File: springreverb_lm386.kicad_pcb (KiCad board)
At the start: 2 copper layers, 65 x 54.7 mm, 50 parts, among them J1 IN, J10 To2, J13 FromGND, J14 From, J15 VR2_3, J16 VR2_3GND, J2 INGND, J3 GND, J4 Vin, J5 VR1_3, J6 VR1_2, J7 VR3_1, J8 ToGND, J9 To, U1 TL072, U2 TC1044S, U3 4556ADD

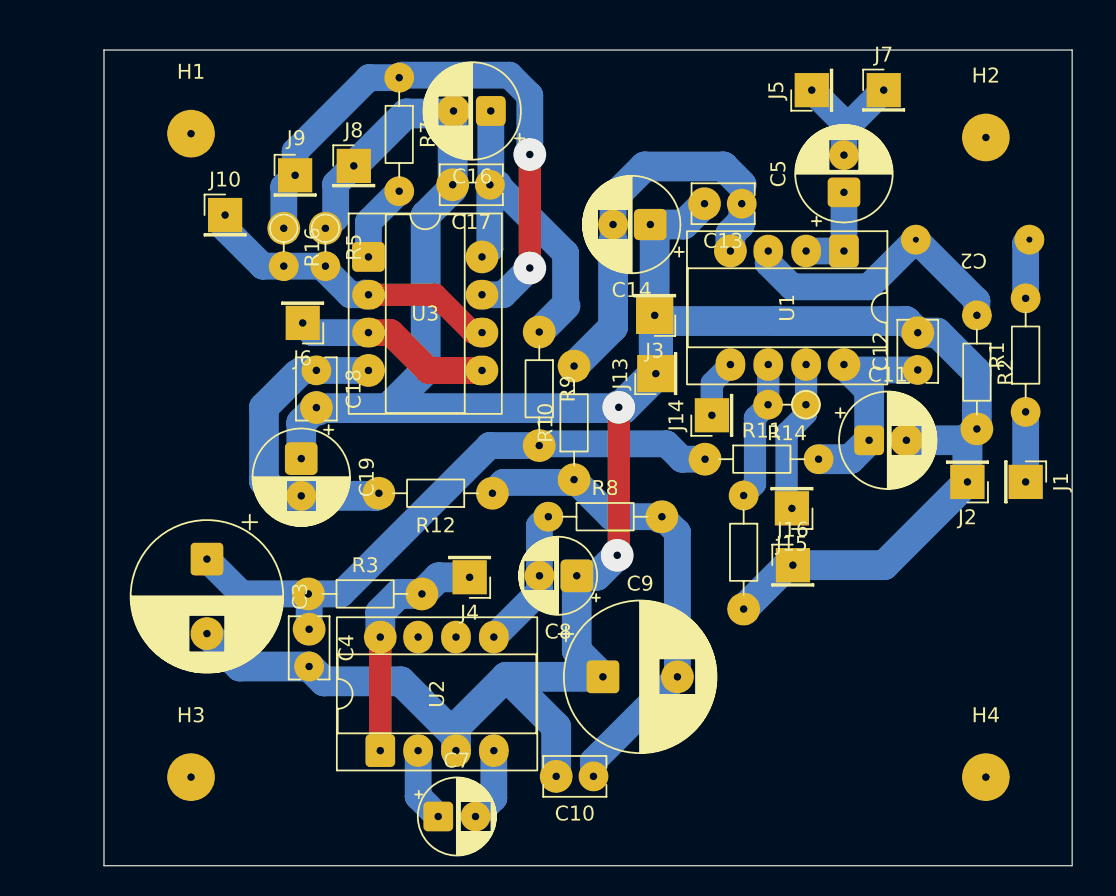
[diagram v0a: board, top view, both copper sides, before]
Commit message: 一旦回路完成
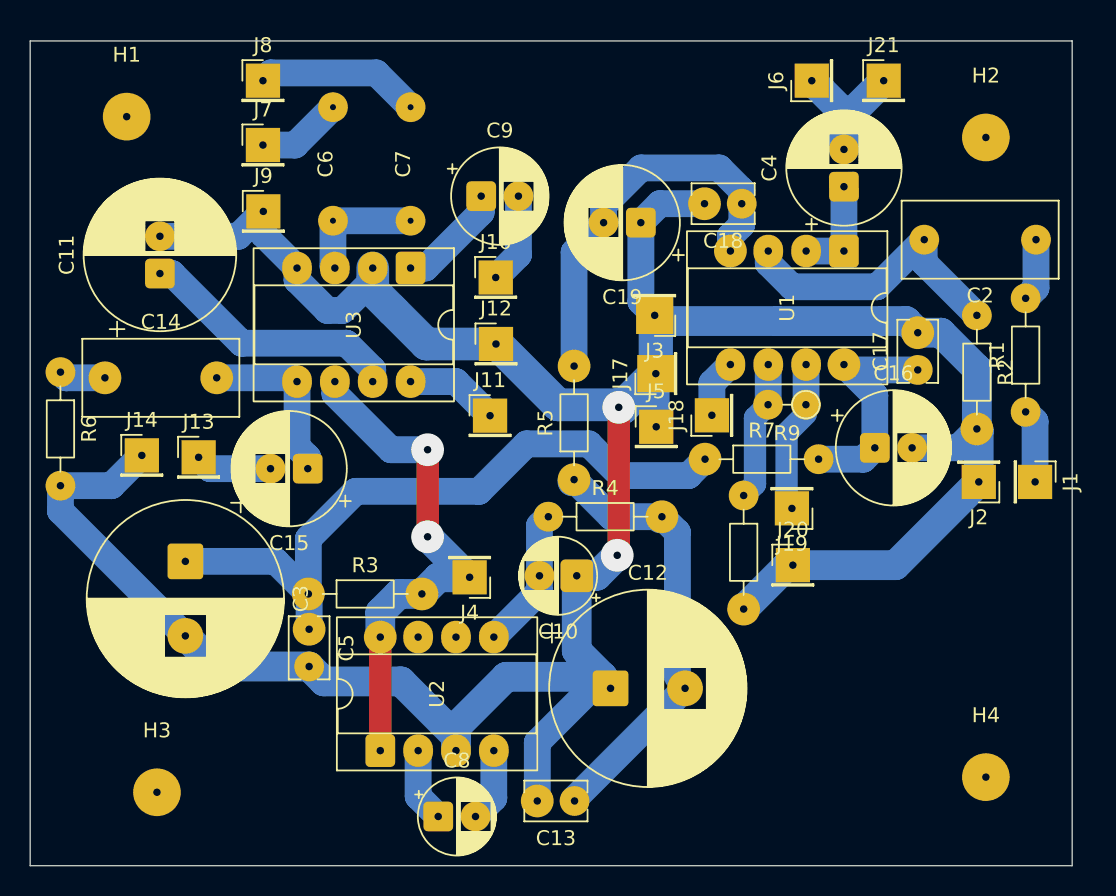
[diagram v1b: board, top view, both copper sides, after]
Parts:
- removed the C16 at (79.8, 70.9)
- removed the C17 at (79.7, 75.8)
- removed the C18 at (68.1, 88.3)
- removed the C19 at (67.1, 94.2)
- removed the J6 at (67.2, 85.1)
- removed R12: 47, Resistor_THT:R_Axial_DIN0204_L3.6mm_D1.6mm_P7.62mm_Horizontal
- removed R16: 1k, Resistor_THT:R_Axial_DIN0204_L3.6mm_D1.6mm_P2.54mm_Vertical
- removed the R5 at (68.7, 78.7)
- removed the R7 at (73.7, 68.6)
- removed the R9 at (83.1, 85.7)
- added C11: 100u, Capacitor_THT:CP_Radial_D10.0mm_P2.50mm, F.Cu at (57.6, 81.8)
- added C14: 0.047u, Capacitor_THT:C_Rect_L10.3mm_W5.0mm_P7.50mm_MKS4, F.Cu at (53.9, 88.8)
- added C15: 100u, Capacitor_THT:CP_Radial_D7.5mm_P2.50mm, F.Cu at (67.5, 94.9)
- added C6: 0.1u, MyLibrary:10.5_5.0_p7.5, F.Cu at (69.2, 74.4)
- added C7: 0.22u, MyLibrary:10.5_5.0_p7.5, F.Cu at (74.4, 74.4)
- added C9: 10u, Capacitor_THT:CP_Radial_D6.3mm_P2.50mm, F.Cu at (79.2, 76.6)
- added J11: VR_2_2, MyLibrary:PinHeader_1x01_P2.54mm_Vertical, F.Cu at (79.8, 91.3)
- added J12: VR_2GND, MyLibrary:PinHeader_1x01_P2.54mm_Vertical, F.Cu at (80.2, 86.5)
- added J13: To, MyLibrary:PinHeader_1x01_P2.54mm_Vertical, F.Cu at (60.2, 94.1)
- added J14: FromSW, MyLibrary:PinHeader_1x01_P2.54mm_Vertical, F.Cu at (56.4, 94.0)
- added J5: LEDGND, MyLibrary:PinHeader_1x01_P2.54mm_Vertical, F.Cu at (90.9, 92.1)
- added J7: toC6, MyLibrary:PinHeader_1x01_P2.54mm_Vertical, F.Cu at (64.5, 73.2)
- added R6: 10, Resistor_THT:R_Axial_DIN0204_L3.6mm_D1.6mm_P7.62mm_Horizontal, F.Cu at (50.9, 88.4)
- C12: renamed from C9; footprint Capacitor_THT:CP_Radial_D10.0mm_P5.00mm -> Capacitor_THT:CP_Radial_D13.0mm_P5.00mm
- C16: renamed from C11; footprint Capacitor_THT:CP_Radial_D6.3mm_P2.50mm -> Capacitor_THT:CP_Radial_D7.5mm_P2.50mm
- C19: renamed from C14; footprint Capacitor_THT:CP_Radial_D6.3mm_P2.50mm -> Capacitor_THT:CP_Radial_D7.5mm_P2.50mm
- C2: footprint MyLibrary:10.5_5.0_p7.5 -> Capacitor_THT:C_Rect_L10.3mm_W5.0mm_P7.50mm_MKS4
- C3: footprint Capacitor_THT:CP_Radial_D10.0mm_P5.00mm -> Capacitor_THT:CP_Radial_D13.0mm_P5.00mm
- C4: renamed from C5; footprint Capacitor_THT:CP_Radial_D6.3mm_P2.50mm -> Capacitor_THT:CP_Radial_D7.5mm_P2.50mm
- J10: value To2 -> VR2_3
- J8: value ToGND -> toC7
- J9: value To -> FromC
- U3: value 4556ADD -> LM386
- moved J10 18.6 mm to (80.1, 82.0)
- moved J8 8.36 mm to (64.5, 68.8)
- moved H1 4.47 mm to (55.4, 71.2)
- moved C2 4.25 mm to (116.4, 79.5)
- moved J9 3.23 mm to (64.5, 77.6)
- moved U3 2.92 mm to (74.4, 81.4), turned to -90 degrees
- moved H3 2.50 mm to (57.4, 116.6)
- moved C13 2.08 mm to (85.4, 117.2)
- moved C3 1.46 mm to (59.3, 101.1)
- moved C12 0.93 mm to (87.8, 109.6)
- moved J2 0.76 mm to (112.6, 95.8)
- moved C19 0.65 mm to (89.9, 78.4)
- moved C16 0.63 mm to (105.6, 93.5)
- moved J1 0.63 mm to (116.3, 95.8)
- moved J21 0.63 mm to (106.2, 68.8)
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- renumbered C8 to C10, C10 to C13, C12 to C17, C13 to C18, C4 to C5, C7 to C8, J13 to J17, J14 to J18, J15 to J19, J16 to J20, J7 to J21, J5 to J6, R8 to R4, R10 to R5, R11 to R7, R13 to R8, R14 to R9
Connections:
- J8 pad 1: GND -> Net-(J8-Pin_1)
- J9 pad 1: Net-(J11-In) -> GND
- U3 pad 2: Net-(J10-Pin_1) -> GND
- U3 pad 3: Net-(J6-Pin_1) -> Net-(U3-+)
- U3 pad 4: Net-(U3C-V-) -> GND
- U3 pad 5: Net-(J6-Pin_1) -> Net-(C14-Pad2)
- U3 pad 6: Net-(J10-Pin_1) -> Net-(J4-Pin_1)
- U3 pad 7: Net-(J11-In) -> Net-(U3-BYPASS)
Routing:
- net Net-(J11-In): track 39.4 -> 0.00 mm, vias 2 -> 0
- net Net-(U3C-V-): track 21.2 -> 0.00 mm
- net Net-(J4-Pin_1): track 16.2 -> 34.6 mm, vias 0 -> 2
- net Net-(U3-BYPASS): track 0.00 -> 17.8 mm
- net Net-(J11-Pin_1): track 23.5 -> 6.28 mm
- net Net-(J10-Pin_1): track 21.8 -> 6.09 mm
- net Net-(J6-Pin_1): track 13.4 -> 0.00 mm
- net Net-(C14-Pad2): track 0.00 -> 11.6 mm
- net Net-(J8-Pin_1): track 0.00 -> 11.1 mm
- net GND: track 194.4 -> 204.9 mm
- net Net-(U3-+): track 0.00 -> 8.43 mm
- net Net-(J7-Pin_1): track 0.00 -> 5.75 mm
- net Net-(J13-Pin_1): track 0.00 -> 5.14 mm
- net Net-(C3-Pad1): track 41.4 -> 45.8 mm
- net Net-(C12-Pad2): track 33.3 -> 29.3 mm
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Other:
- board size 65 x 54.7 mm -> 69.9 x 55.3 mm
